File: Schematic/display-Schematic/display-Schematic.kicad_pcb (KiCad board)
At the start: 2 copper layers, 197.7 x 46 mm, 31 parts, among them SW1 up, SW2 left, SW3 left, SW4 down, SW5 setup, U10 5161AS, U11 5161AS, U12 5161AS, U13 5161AS, U4 MAX7219, U5 12101AR, U6 12101AR, U7 12101AR, U8 12101AR, U9 MAX7219

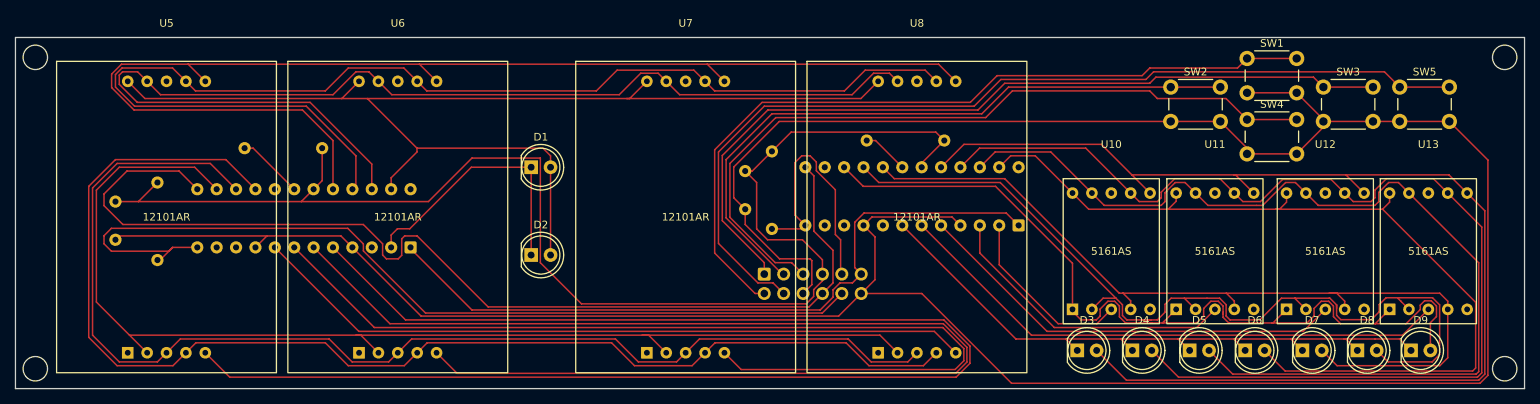
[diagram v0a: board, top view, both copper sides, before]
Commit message: Further work on the hardware side of the pcb
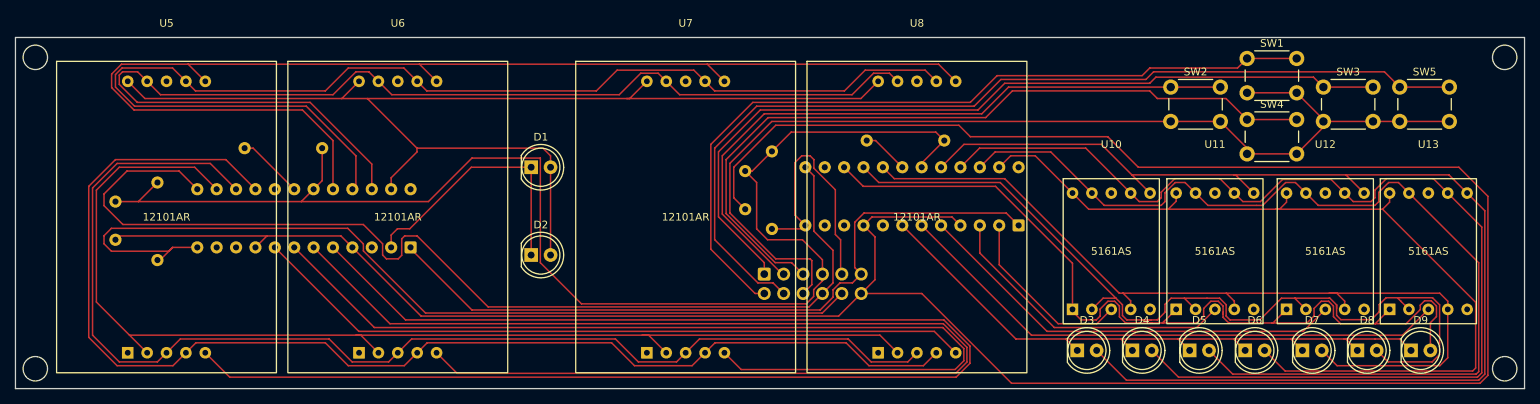
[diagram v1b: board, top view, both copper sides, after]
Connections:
- J1 pad 6: GND -> +3.3V
- SW1 pad 2: GND -> +3.3V
- SW2 pad 2: GND -> +3.3V
- SW3 pad 2: GND -> +3.3V
- SW4 pad 2: GND -> +3.3V
- SW5 pad 2: GND -> +3.3V
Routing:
- net +3.3V: track 0.00 -> 138.0 mm
- net GND: track 389.0 -> 351.4 mm
- net Net-(SW1A-C): track 103.4 -> 104.6 mm
- net Net-(SW5A-C): track 124.2 -> 125.2 mm
- net Net-(SW4A-C): track 99.5 -> 100.5 mm
- net Net-(SW2A-C): track 86.9 -> 87.9 mm
- net Net-(SW3A-C): track 107.9 -> 108.8 mm
